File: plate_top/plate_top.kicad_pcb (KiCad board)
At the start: 2 copper layers, 157.5 x 118.1 mm, 31 parts, among them SW1 SW_Push

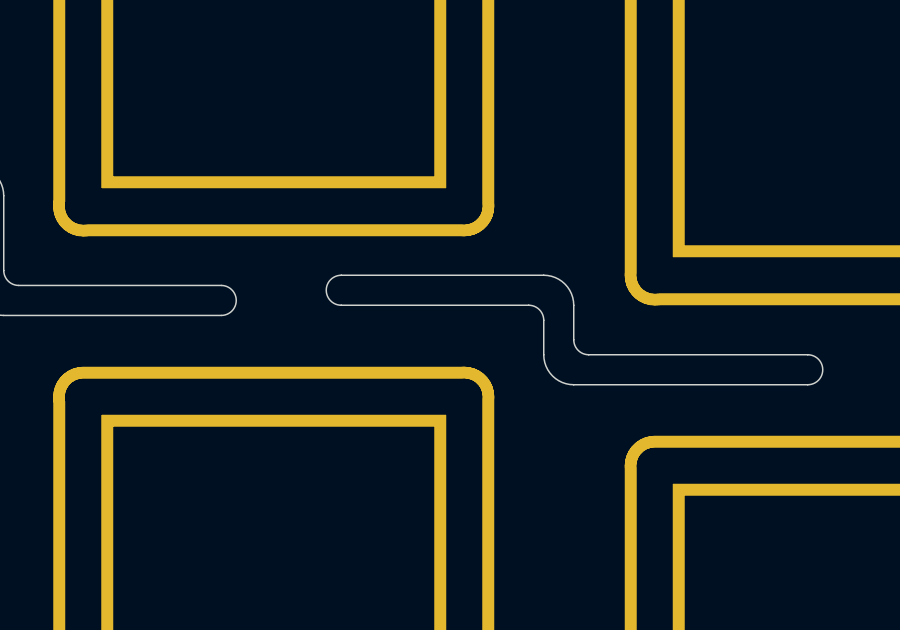
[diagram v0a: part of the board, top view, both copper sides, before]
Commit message: Cuts
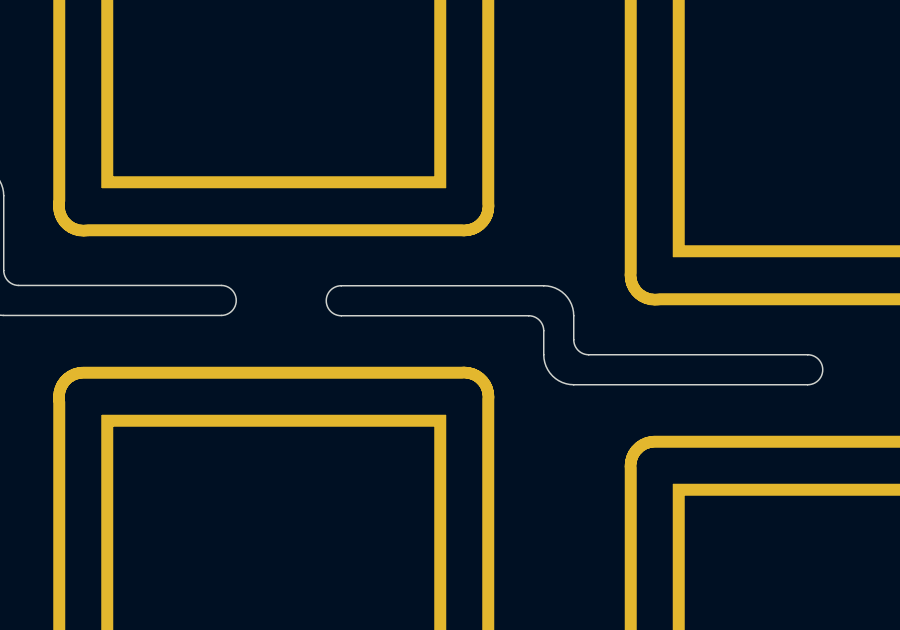
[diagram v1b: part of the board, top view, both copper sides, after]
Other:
- outline, holes or cut-outs redrawn
